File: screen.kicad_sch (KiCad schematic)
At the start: 11 parts, among them J4 Screen FPC, Q1 NMOS

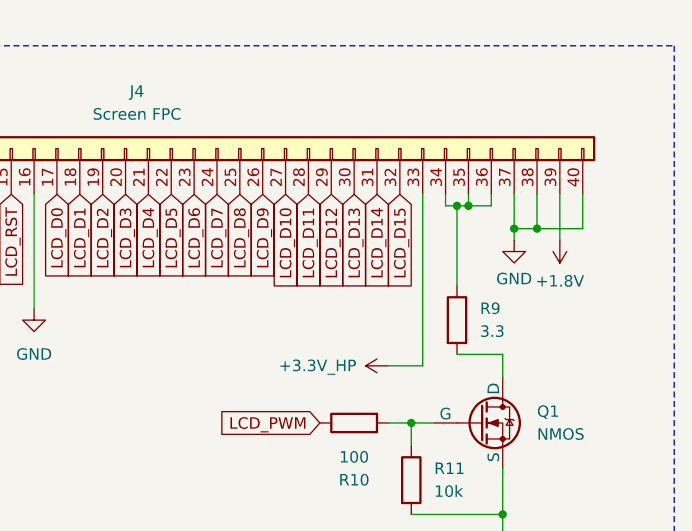
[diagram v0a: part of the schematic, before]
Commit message: pcb draft, cleaned up schematic
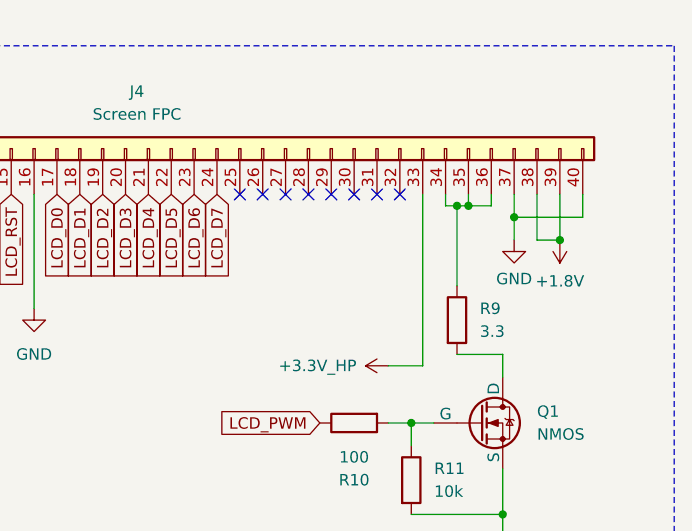
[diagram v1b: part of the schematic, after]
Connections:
- net +1.8V: now also J4.38 (Pin_38)
- net GND: no longer J4.38 (Pin_38)
- net LCD_D10: no longer names the net of J4.27 (Pin_27)
- net LCD_D11: no longer names the net of J4.28 (Pin_28)
- net LCD_D12: no longer names the net of J4.29 (Pin_29)
- net LCD_D13: no longer names the net of J4.30 (Pin_30)
- net LCD_D14: no longer names the net of J4.31 (Pin_31)
- net LCD_D15: no longer names the net of J4.32 (Pin_32)
- net LCD_D8: no longer names the net of J4.25 (Pin_25)
- net LCD_D9: no longer names the net of J4.26 (Pin_26)
- no-connect marks 3 -> 11
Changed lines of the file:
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@@
-	)
-	(junction
-		(at 190.5 71.12)
-		(diameter 0)
-		(color 0 0 0 0)
 	)
 	(junction
@@
 	)
 	(junction
+		(at 195.58 72.39)
+		(diameter 0)
+		(color 0 0 0 0)
+	)
+	(junction
 		(at 179.07 92.71)
 		(diameter 0)
@@
 	)
 	(junction
+		(at 190.5 69.85)
+		(diameter 0)
+		(color 0 0 0 0)
+	)
+	(junction
 		(at 121.92 120.65)
 		(diameter 0)
@@
 	)
 	(junction
-		(at 193.04 71.12)
-		(diameter 0)
-		(color 0 0 0 0)
-	)
-	(junction
 		(at 111.76 81.28)
 		(diameter 0)
@@
 	)
 	(no_connect
+		(at 167.64 67.31)
+	)
+	(no_connect
+		(at 172.72 67.31)
+	)
+	(no_connect
 		(at 129.54 67.31)
 	)
 	(no_connect
+		(at 160.02 67.31)
+	)
+	(no_connect
+		(at 170.18 67.31)
+	)
+	(no_connect
+		(at 177.8 67.31)
+	)
+	(no_connect
 		(at 132.08 67.31)
 	)
@@
 		(at 116.84 67.31)
 	)
+	(no_connect
+		(at 162.56 67.31)
+	)
+	(no_connect
+		(at 175.26 67.31)
+	)
+	(no_connect
+		(at 165.1 67.31)
+	)
 	(wire
 		(pts
@@
 	(wire
 		(pts
-			(xy 193.04 71.12) (xy 193.04 67.31)
-		)
-		(stroke
-			(width 0)
-			(type default)
-		)
-	)
-	(wire
-		(pts
 			(xy 106.68 67.31) (xy 106.68 69.85)
 		)
@@
 	(wire
 		(pts
+			(xy 195.58 67.31) (xy 195.58 72.39)
+		)
+		(stroke
+			(width 0)
+			(type default)
+		)
+	)
+	(wire
+		(pts
 			(xy 137.16 67.31) (xy 137.16 80.01)
 		)
@@
 	(wire
 		(pts
-			(xy 190.5 71.12) (xy 193.04 71.12)
-		)
-		(stroke
-			(width 0)
-			(type default)
-		)
-	)
-	(wire
-		(pts
 			(xy 189.23 85.09) (xy 189.23 87.63)
 		)
@@
 	(wire
 		(pts
+			(xy 198.12 69.85) (xy 190.5 69.85)
+		)
+		(stroke
+			(width 0)
+			(type default)
+		)
+	)
+	(wire
+		(pts
 			(xy 99.06 67.31) (xy 99.06 81.28)
 		)
@@
 	(wire
 		(pts
-			(xy 198.12 67.31) (xy 198.12 71.12)
-		)
-		(stroke
-			(width 0)
-			(type default)
-		)
-	)
-	(wire
-		(pts
-			(xy 195.58 67.31) (xy 195.58 72.39)
-		)
-		(stroke
-			(width 0)
-			(type default)
-		)
-	)
-	(wire
-		(pts
 			(xy 121.92 102.87) (xy 121.92 120.65)
 		)
@@
 	(wire
 		(pts
+			(xy 198.12 67.31) (xy 198.12 69.85)
+		)
+		(stroke
+			(width 0)
+			(type default)
+		)
+	)
+	(wire
+		(pts
 			(xy 93.98 69.85) (xy 93.98 101.6)
 		)
@@
 	(wire
 		(pts
+			(xy 193.04 72.39) (xy 195.58 72.39)
+		)
+		(stroke
+			(width 0)
+			(type default)
+		)
+	)
+	(wire
+		(pts
 			(xy 180.34 86.36) (xy 176.53 86.36)
 		)
@@
 	(wire
 		(pts
-			(xy 190.5 67.31) (xy 190.5 71.12)
-		)
-		(stroke
-			(width 0)
-			(type default)
-		)
-	)
-	(wire
-		(pts
 			(xy 109.22 102.87) (xy 109.22 123.19)
 		)
@@
 	(wire
 		(pts
-			(xy 198.12 71.12) (xy 193.04 71.12)
-		)
-		(stroke
-			(width 0)
-			(type default)
-		)
-	)
-	(wire
-		(pts
 			(xy 179.07 102.87) (xy 189.23 102.87)
 		)
@@
 	(wire
 		(pts
-			(xy 190.5 71.12) (xy 190.5 72.39)
+			(xy 190.5 69.85) (xy 190.5 72.39)
+		)
+		(stroke
+			(width 0)
+			(type default)
+		)
+	)
+	(wire
+		(pts
+			(xy 190.5 67.31) (xy 190.5 69.85)
+		)
+		(stroke
+			(width 0)
+			(type default)
+		)
+	)
+	(wire
+		(pts
+			(xy 193.04 67.31) (xy 193.04 72.39)
 		)
 		(stroke
@@
 		)
 	)
-	(global_label "LCD_D12"
-		(shape input)
-		(at 170.18 67.31 270)
-		(fields_autoplaced yes)
-		(effects
-			(font
-				(size 1.27 1.27)
-			)
-			(justify right)
-		)
-		(property "Intersheetrefs" "${INTERSHEET_REFS}"
-			(at 170.18 77.3104 90)
-			(hide yes)
-			(show_name no)
-			(do_not_autoplace no)
-			(effects
-				(font
-					(size 1.27 1.27)
-				)
-				(justify right)
-			)
-		)
-	)
 	(global_label "LCD_NE1"
 		(shape input)
@@
 		)
 	)
-	(global_label "LCD_D15"
-		(shape input)
-		(at 177.8 67.31 270)
-		(fields_autoplaced yes)
-		(effects
-			(font
-				(size 1.27 1.27)
-			)
-			(justify right)
-		)
-		(property "Intersheetrefs" "${INTERSHEET_REFS}"
-			(at 177.8 77.3104 90)
-			(hide yes)
-			(show_name no)
-			(do_not_autoplace no)
-			(effects
-				(font
-					(size 1.27 1.27)
-				)
-				(justify right)
-			)
-		)
-	)
 	(global_label "CTP_INT"
 		(shape input)
@@
 		)
 	)
-	(global_label "LCD_D10"
-		(shape input)
-		(at 165.1 67.31 270)
-		(fields_autoplaced yes)
-		(effects
-			(font
-				(size 1.27 1.27)
-			)
-			(justify right)
-		)
-		(property "Intersheetrefs" "${INTERSHEET_REFS}"
-			(at 165.1 77.3104 90)
-			(hide yes)
-			(show_name no)
-			(do_not_autoplace no)
-			(effects
-				(font
-					(size 1.27 1.27)
-				)
-				(justify right)
-			)
-		)
-	)
 	(global_label "LCD_D7"
 		(shape input)
@@
 		)
 	)
-	(global_label "LCD_D11"
-		(shape input)
-		(at 167.64 67.31 270)
-		(fields_autoplaced yes)
-		(effects
-			(font
-				(size 1.27 1.27)
-			)
-			(justify right)
-		)
-		(property "Intersheetrefs" "${INTERSHEET_REFS}"
-			(at 167.64 77.3104 90)
-			(hide yes)
-			(show_name no)
-			(do_not_autoplace no)
-			(effects
-				(font
-					(size 1.27 1.27)
-				)
-				(justify right)
-			)
-		)
-	)
 	(global_label "CTP_SCL"
 		(shape input)
@@
 		)
 	)
-	(global_label "LCD_D13"
-		(shape input)
-		(at 172.72 67.31 270)
-		(fields_autoplaced yes)
-		(effects
-			(font
-				(size 1.27 1.27)
-			)
-			(justify right)
-		)
-		(property "Intersheetrefs" "${INTERSHEET_REFS}"
-			(at 172.72 77.3104 90)
-			(hide yes)
-			(show_name no)
-			(do_not_autoplace no)
-			(effects
-				(font
-					(size 1.27 1.27)
-				)
-				(justify right)
-			)
-		)
-	)
 	(global_label "LCD_D0"
 		(shape input)
@@
 		)
 	)
-	(global_label "LCD_D9"
-		(shape input)
-		(at 162.56 67.31 270)
-		(fields_autoplaced yes)
-		(effects
-			(font
-				(size 1.27 1.27)
-			)
-			(justify right)
-		)
-		(property "Intersheetrefs" "${INTERSHEET_REFS}"
-			(at 162.56 77.3104 90)
-			(hide yes)
-			(show_name no)
-			(do_not_autoplace no)
-			(effects
-				(font
-					(size 1.27 1.27)
-				)
-				(justify right)
-			)
-		)
-	)
 	(global_label "LCD_D2"
 		(shape input)
@@
 		)
 	)
-	(global_label "LCD_D14"
-		(shape input)
-		(at 175.26 67.31 270)
-		(fields_autoplaced yes)
-		(effects
-			(font
-				(size 1.27 1.27)
-			)
-			(justify right)
-		)
-		(property "Intersheetrefs" "${INTERSHEET_REFS}"
-			(at 175.26 77.3104 90)
-			(hide yes)
-			(show_name no)
-			(do_not_autoplace no)
-			(effects
-				(font
-					(size 1.27 1.27)
-				)
-				(justify right)
-			)
-		)
-	)
 	(global_label "LCD_RS"
 		(shape input)
@@
 			(hide yes)
 			(show_name no)
-			(do_not_autoplace no)
-			(effects
-				(font
-					(size 1.27 1.27)
-				)
-				(justify right)
-			)
-		)
-	)
-	(global_label "LCD_D8"
-		(shape input)
-		(at 160.02 67.31 270)
-		(fields_autoplaced yes)
-		(effects
-			(font
-				(size 1.27 1.27)
-			)
-			(justify right)
-		)
-		(property "Intersheetrefs" "${INTERSHEET_REFS}"
-			(at 160.02 77.3104 90)
-			(hide yes)
-			(show_name no)
